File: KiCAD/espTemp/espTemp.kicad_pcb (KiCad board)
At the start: 2 copper layers, 39.4 x 24.8 mm, 7 parts, among them U1 ESP-01, U2 LD1117S33TR_SOT223, U3 DHT11

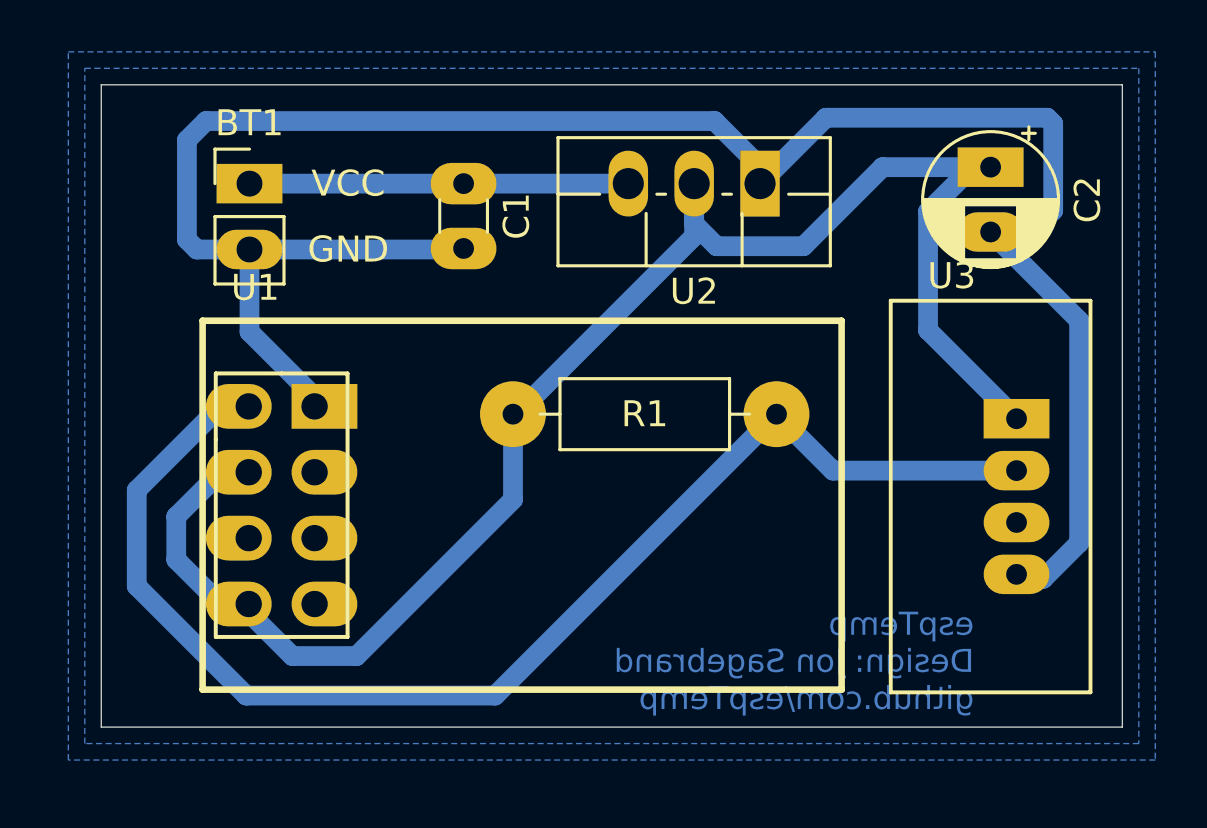
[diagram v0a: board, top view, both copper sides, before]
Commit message: kicad
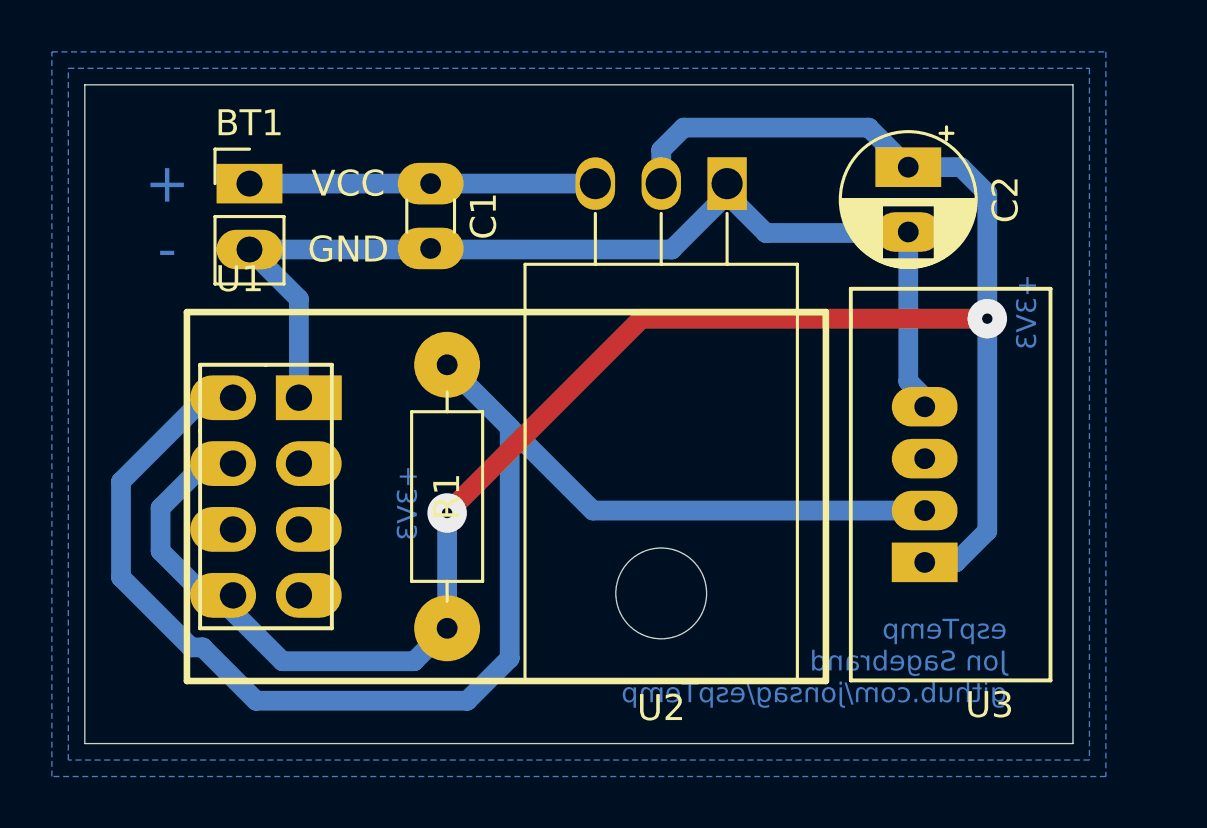
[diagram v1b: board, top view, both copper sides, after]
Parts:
- U2: footprint My_Parts:TO-220F-3_Vertical_large -> My_Misc:TO-220F-3_Horizontal_TabDown_large
- moved R1 8.64 mm to (146.1, 94.0), turned to 90 degrees
- moved C2 3.17 mm to (163.8, 76.2)
- moved U3 1.61 mm to (165.5, 88.4), turned to 180 degrees
- moved C1 1.27 mm to (145.4, 76.8)
- moved U2 1.27 mm to (156.8, 76.8)
- moved U1 0.69 mm to (137.8, 85.1)
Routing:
- net GND: track 80.5 -> 40.0 mm
- net +3V3: track 64.2 -> 78.1 mm, vias 0 -> 2
- net GPIO1: track 50.0 -> 60.0 mm
- net Net-(BT1-Pad1): track 14.6 -> 13.3 mm
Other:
- board size 39.4 x 24.8 mm -> 38.1 x 25.4 mm
- net class Default: via_dia 0.8 -> 1.524
- board text added: "+"
- board text added: "+3V3"
- board text added: "-"
- board text added: "espTemp Jon Sagebrand github.com/jonsag/espTemp"
- board text removed: "espTemp Design: Jon Sagebrand github.com/espTemp"
